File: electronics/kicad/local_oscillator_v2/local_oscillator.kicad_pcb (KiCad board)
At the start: 2 copper layers, 29 parts, among them P1 TestPoint:TestPoint_Pad_1.5x1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, P2 TestPoint:TestPoint_Pad_1.5x1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, P3 TestPoint:TestPoint_Pad_1.5x1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, P4 TestPoint:TestPoint_Pad_1.5x1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, P5 TestPoint:TestPoint_Pad_1.5x1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, P6 TestPoint:TestPoint_Pad_1.5x1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, Q1 BSS138, Q2 BSS138, U1 CE3520K3

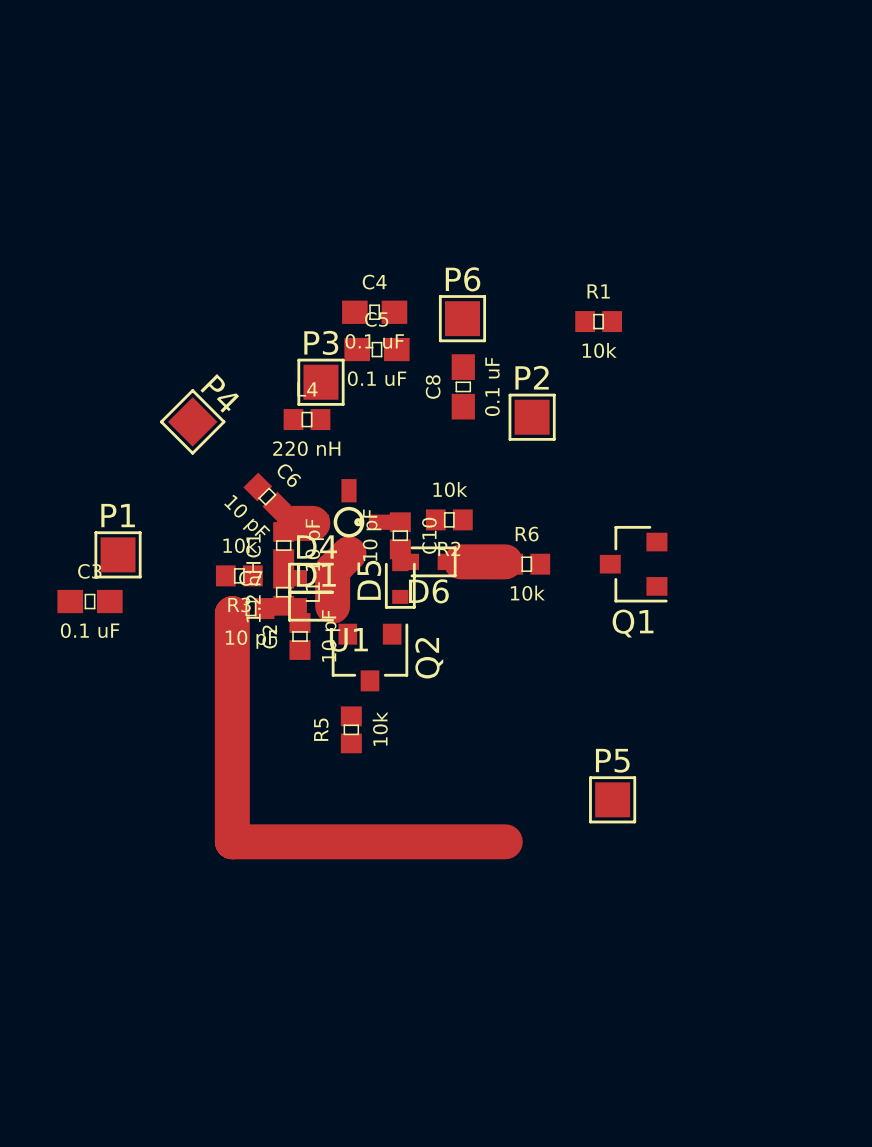
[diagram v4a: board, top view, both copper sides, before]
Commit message: LO test something more
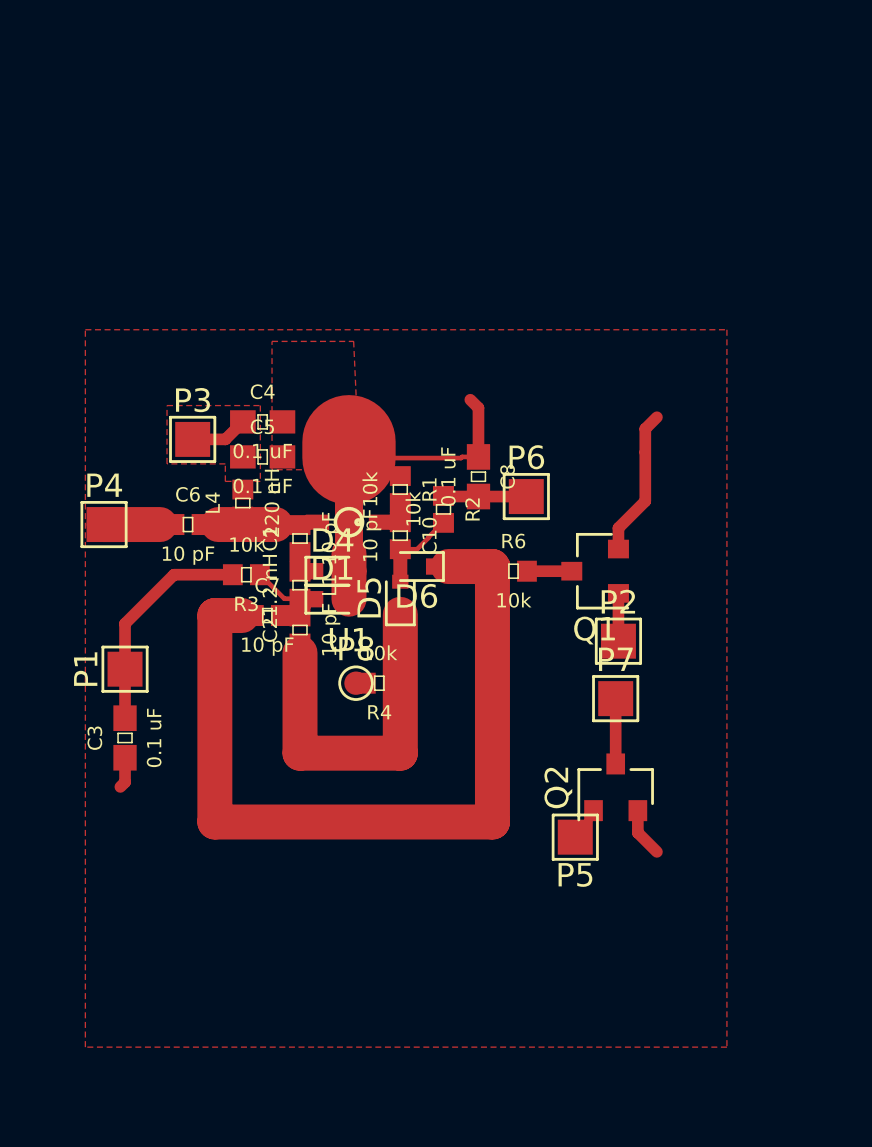
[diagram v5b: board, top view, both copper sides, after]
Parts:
- removed R5: 10k, Capacitors:0402
- added P7: TestPoint:TestPoint_Pad_1.5x1.5mm, TestPoint:TestPoint_Pad_1.5x1.5mm, F.Cu at (82.0, 55.5)
- added P8: TestPoint:TestPoint_Pad_1.5x1.5mm, TestPoint:TestPoint_Pad_D1.0mm, F.Cu at (70.9, 54.8)
- added R4: 10k, Capacitors:0402, F.Cu at (71.9, 54.8)
- moved Q2 11.9 mm to (82.0, 59.3), turned to 90 degrees
- moved R1 11.1 mm to (72.8, 46.5), turned to 270 degrees
- moved P2 10.3 mm to (82.2, 53.0)
- moved P6 8.10 mm to (78.2, 46.8)
- moved C5 6.72 mm to (66.9, 45.1)
- moved C4 6.72 mm to (66.9, 43.6)
- moved C3 6.04 mm to (61.0, 57.1), turned to 90 degrees
- moved P3 6.02 mm to (63.9, 44.4)
- moved P4 5.81 mm to (60.1, 48.0), turned to 0 degrees
- moved P1 4.91 mm to (61.0, 54.2), turned to 90 degrees
- moved L4 4.51 mm to (66.0, 47.1), turned to 90 degrees
- moved C8 3.90 mm to (76.2, 46.0), turned to 270 degrees
- moved C6 3.61 mm to (63.7, 48.0), turned to 0 degrees
- moved P5 2.26 mm to (80.3, 61.4), turned to 180 degrees
- moved Q1 1.68 mm to (81.2, 50.0)
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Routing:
- net GND: track 2.54 -> 24.0 mm
- net Net-(C2-Pad1): track 0.00 -> 14.5 mm
- net Net-(C7-Pad1): track 23.4 -> 34.8 mm
- net Net-(C3-Pad2): track 0.00 -> 9.54 mm
- net Net-(C8-Pad2): track 0.00 -> 3.60 mm
- net Net-(P7-Pad1): track 0.00 -> 2.80 mm
- net Net-(C4-Pad1): track 0.00 -> 2.46 mm
- net Net-(C6-Pad1): track 0.00 -> 2.40 mm
- net Net-(C10-Pad2): track 0.00 -> 2.33 mm
- net Net-(C2-Pad2): track 0.00 -> 2.15 mm
- net Net-(P2-Pad1): track 0.00 -> 2.05 mm
- net Net-(Q1-Pad3): track 0.00 -> 1.92 mm
- net /VCC: track 0.80 -> 2.45 mm
- added copper zone on F.Cu, net GND
- added copper zone on F.Cu, net Net-(C4-Pad1)
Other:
- net class Default: trace_width 1.5 -> 0.5
